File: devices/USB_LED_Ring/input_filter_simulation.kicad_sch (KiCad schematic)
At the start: 24 parts

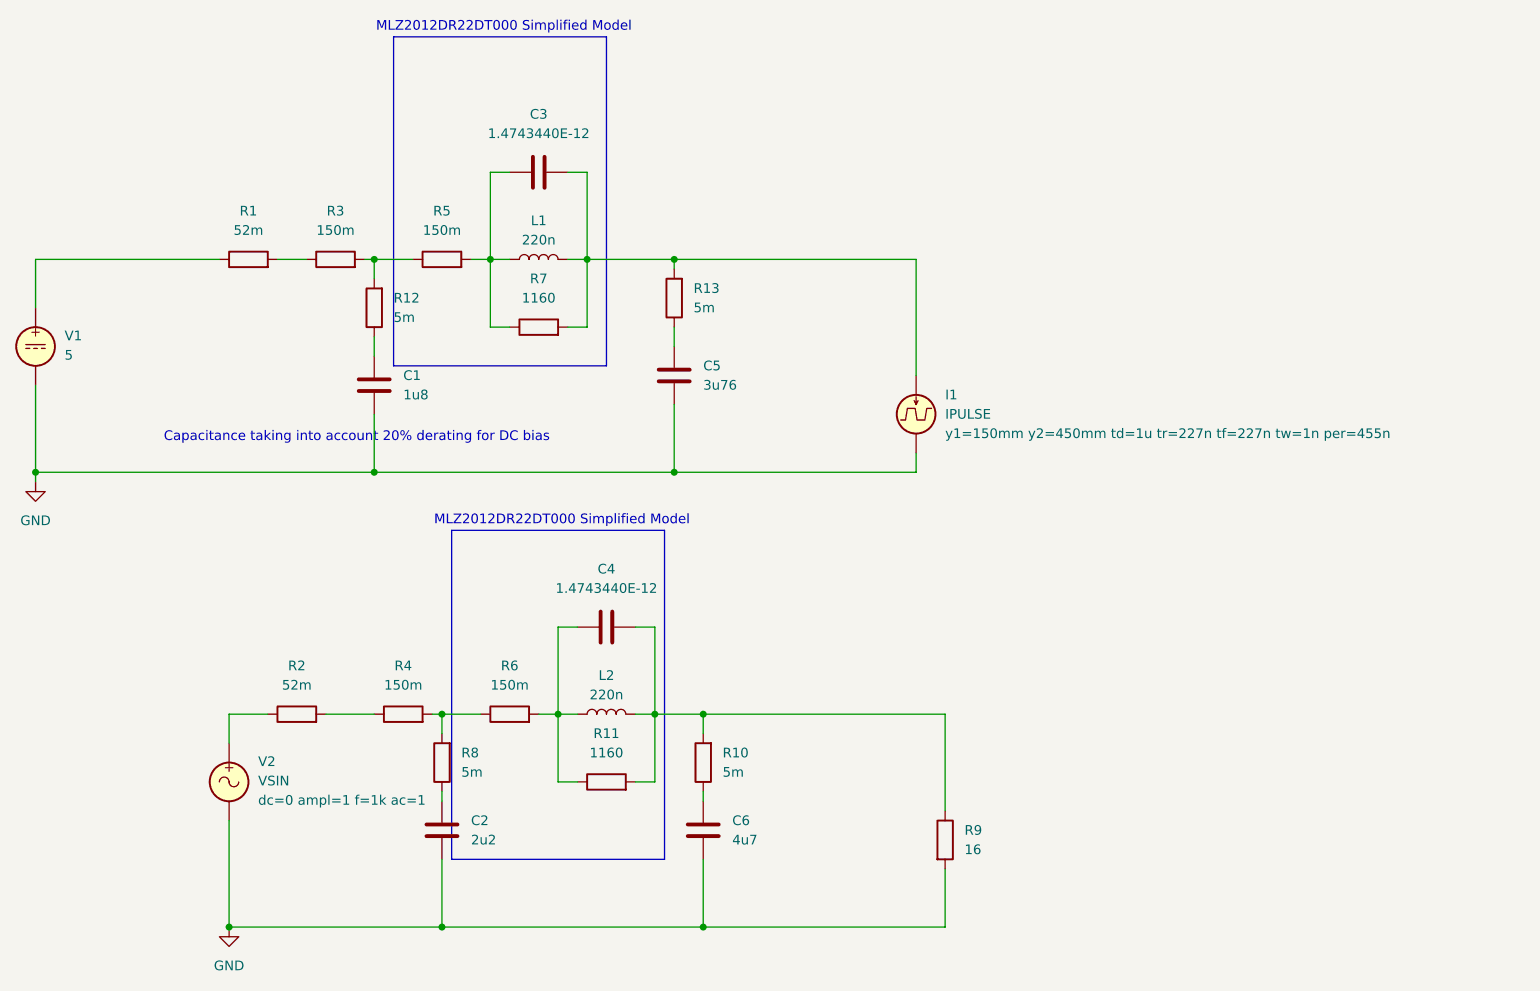
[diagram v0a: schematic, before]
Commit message: !fixup
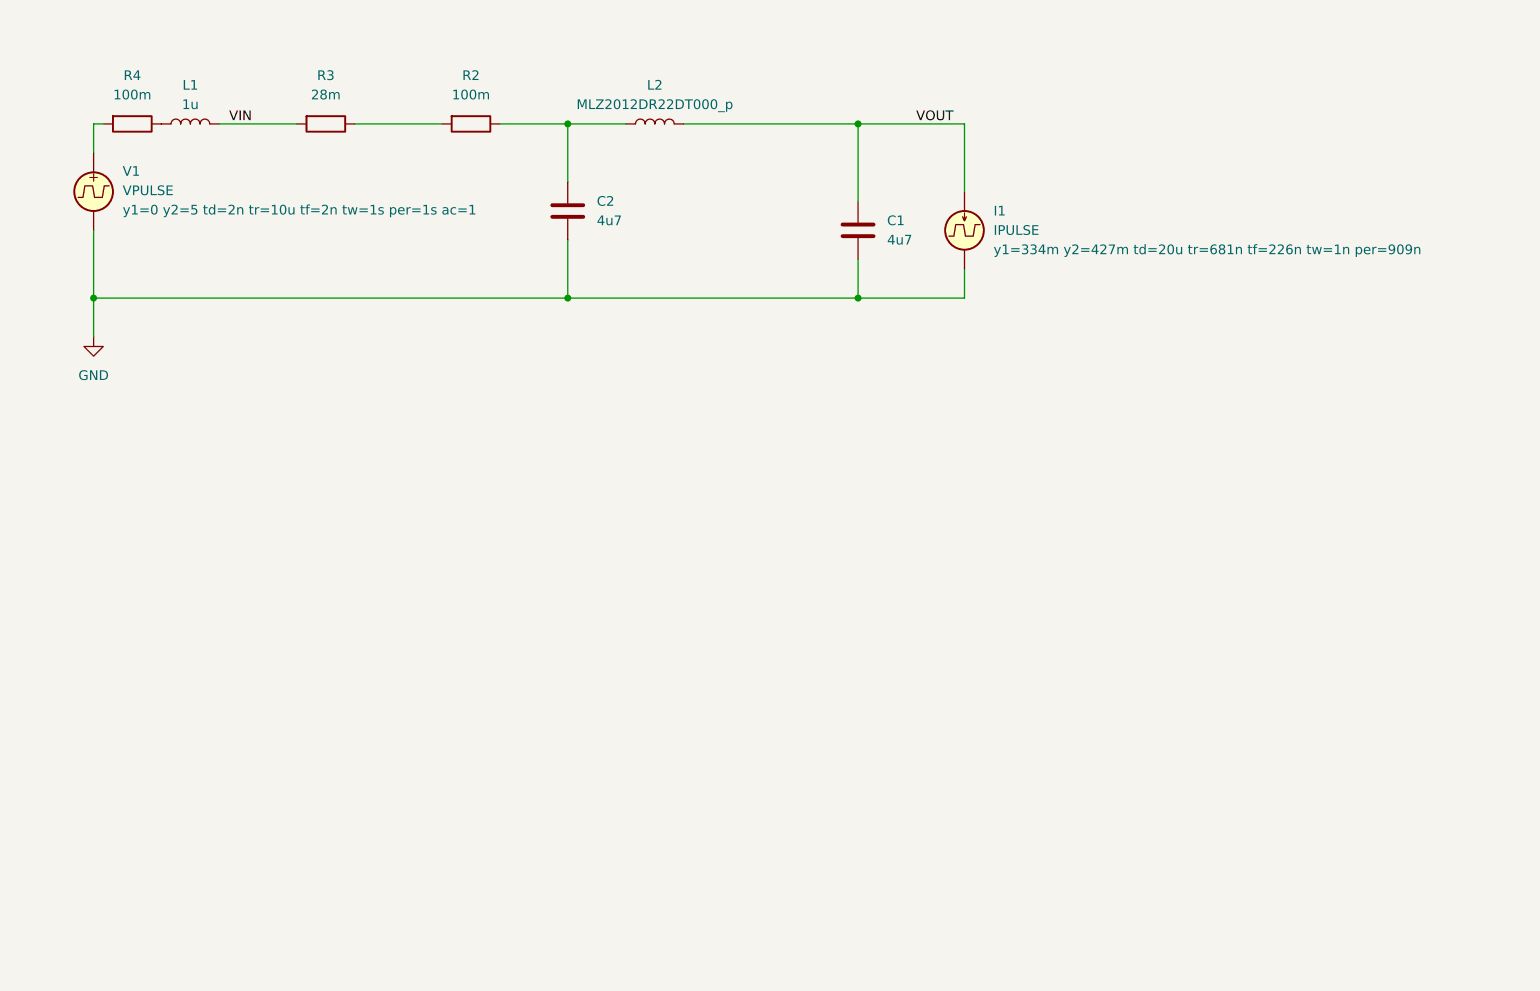
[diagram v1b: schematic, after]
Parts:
- removed C1: 1u8, symbol Device:C
- removed C3, C4: 1.4743440E-12, symbol Device:C
- removed C5: 3u76, symbol Device:C
- removed R1: 52m, symbol Device:R
- removed R10, R12, R13, R8: 5m, symbol Device:R
- removed R11, R7: 1160, symbol Device:R
- removed R5, R6: 150m, symbol Device:R
- removed R9: 16, symbol Device:R
- removed V1: 5, symbol Simulation_SPICE:VDC
- removed V2: VSIN, symbol Simulation_SPICE:VSIN
- added V1: VPULSE, symbol Simulation_SPICE:VPULSE
- C2: value 2u2 -> 4u7
- L1: value 220n -> 1u
- L2: value 220n -> ${SIM.PARAMS}
- R2: value 52m -> 100m
- R3: value 150m -> 28m
- R4: value 150m -> 100m
- renumbered C6 to C1
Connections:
- net GND: now also V1.2
- net at L1.1: now also R4.1
- net VIN: now reaches L1.2
- net VIN: now also R3.2; no longer I1.1
- net at R4.2: now also V1.1
- net at L2.1: now also C2.1, R2.1
- net VOUT: now reaches L2.2
- net VOUT: now also C1.1, I1.1
- net at R2.2: now also R3.1; no longer R4.1
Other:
- note removed: "Capacitance taking into account 20% derating for DC bias"
- note removed: "MLZ2012DR22DT000 Simplified Model"
- moved on the sheet: C1
